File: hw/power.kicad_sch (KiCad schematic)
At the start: 20 parts, among them J4 Prog/debug, Q4 AO3401A, Q5 8205A, U2 TP4057, U3 AP7361C-25ER-13, U4 DW01A

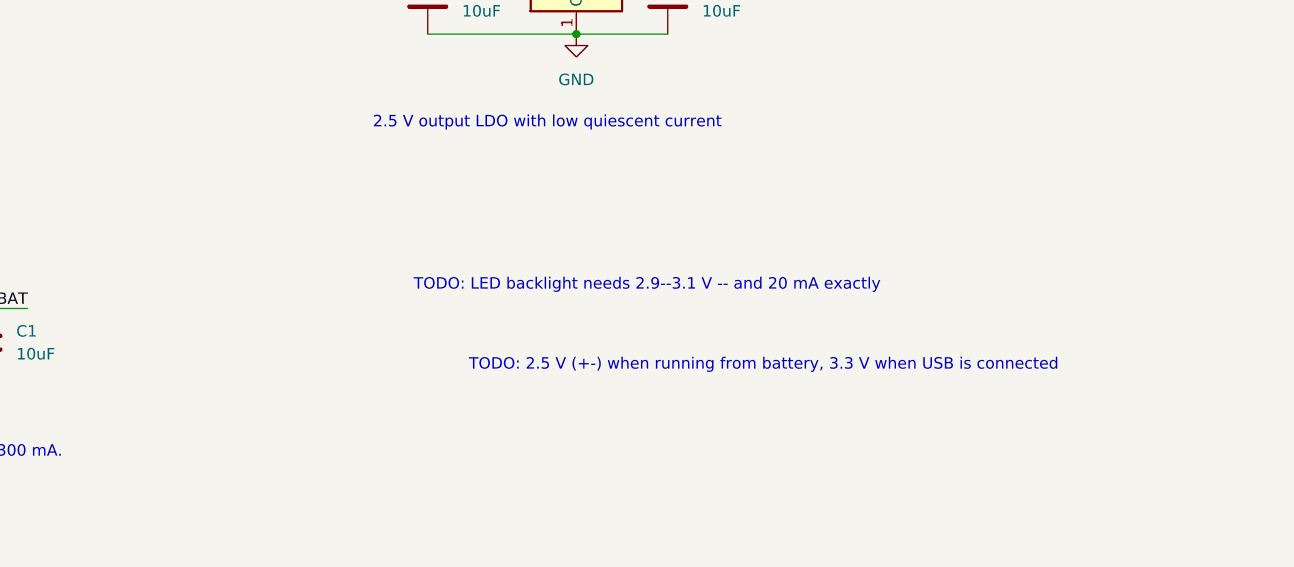
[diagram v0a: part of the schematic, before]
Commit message: WIP
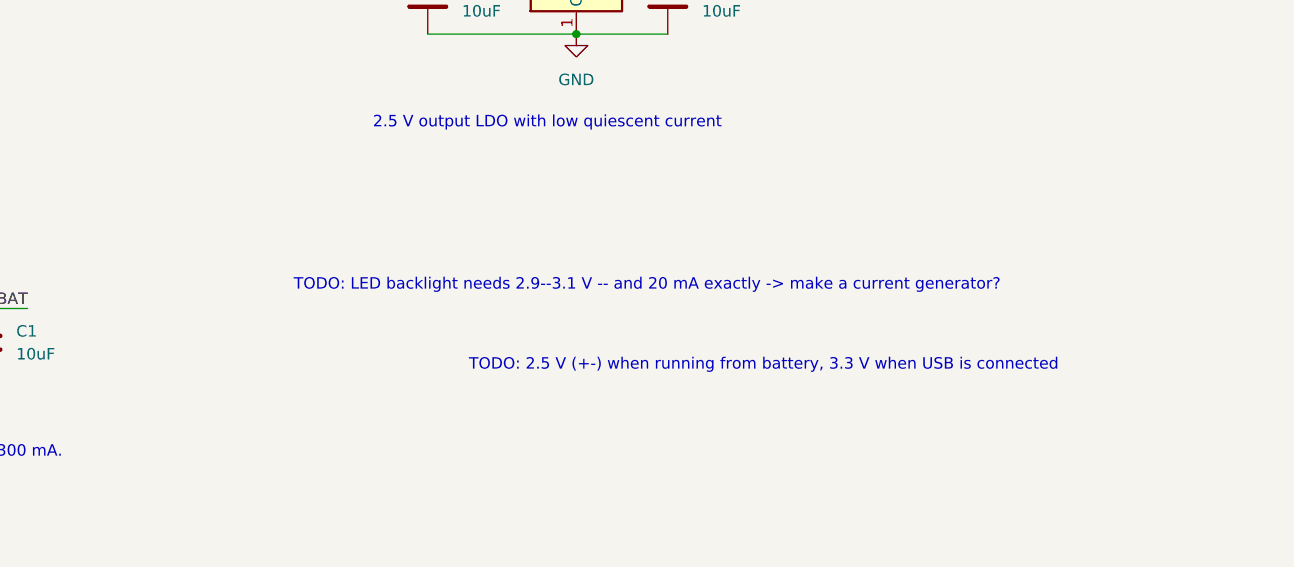
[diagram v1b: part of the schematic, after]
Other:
- note added: "TODO: LED backlight needs 2.9--3.1 V -- and 20 mA exactly -> make a current generator?"
- note removed: "TODO: LED backlight needs 2.9--3.1 V -- and 20 mA exactly"
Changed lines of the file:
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@@
 		)
 	)
-	(text "TODO: LED backlight needs 2.9--3.1 V -- and 20 mA exactly"
+	(text "TODO: LED backlight needs 2.9--3.1 V -- and 20 mA exactly -> make a current generator?"
 		(exclude_from_sim no)
 		(at 175.514 68.58 0)
